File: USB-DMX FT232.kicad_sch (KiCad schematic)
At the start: 26 parts, among them J1 USB, J2 NC3MAFH-PH, U1 FT232RL, U2 TEA1-0505, U3 6N137, U4 MAX485E

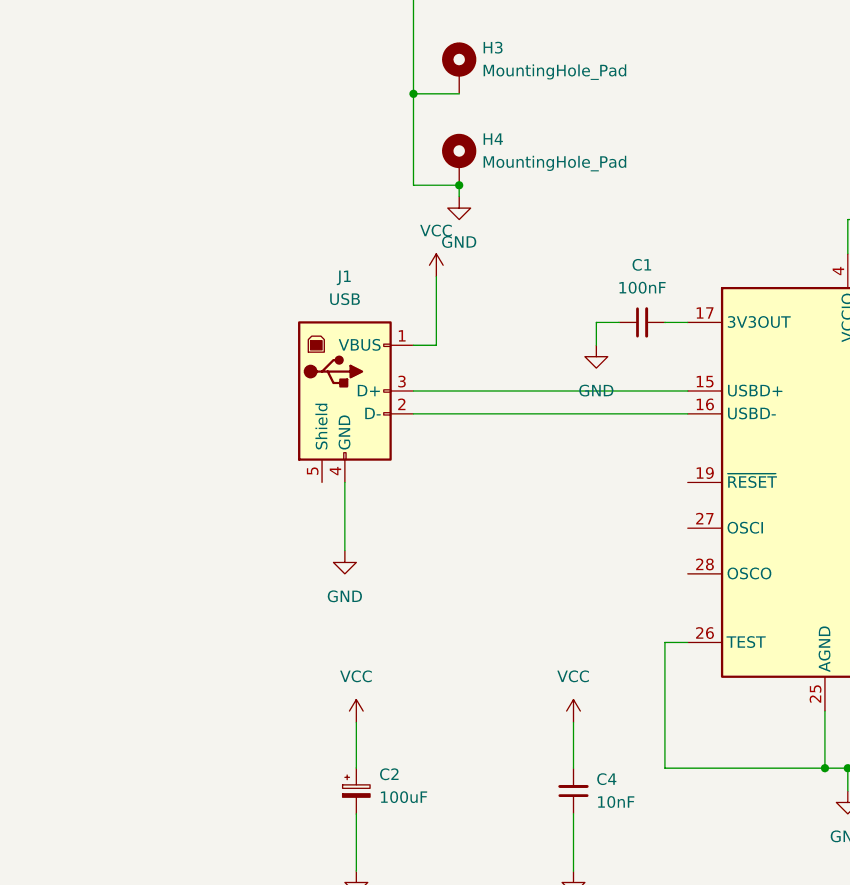
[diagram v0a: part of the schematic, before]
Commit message: usbc version
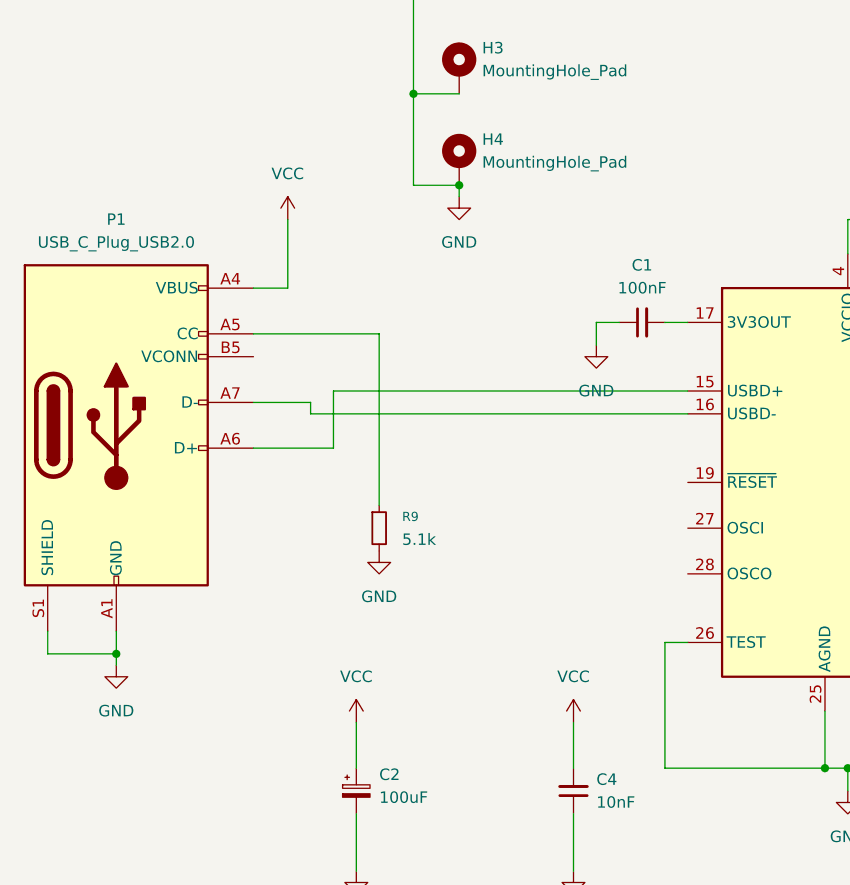
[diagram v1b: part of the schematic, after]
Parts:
- removed J1: USB, Connector_USB:USB_B_Lumberg_2411_02_Horizontal, symbol Connector:USB_B
- added P1: USB_C_Plug_USB2.0, Connector_USB:USB_C_Receptacle_JAE_DX07S016JA1R1500, symbol Connector:USB_C_Plug_USB2.0
- added R9: 5.1k, Resistor_SMD:R_0805_2012Metric_Pad1.20x1.40mm_HandSolder, symbol Device:R_Small
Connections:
- net GND: now also P1.A1 (GND), P1.A12 (GND), P1.B1 (GND), P1.B12 (GND), P1.S1 (SHIELD), R9.2
- net VCC: now also P1.A4 (VBUS), P1.A9 (VBUS), P1.B4 (VBUS), P1.B9 (VBUS)
- net at U1.16 (USBD-): now also P1.A7 (D-)
- net at U1.15 (USBD+): now also P1.A6 (D+)
- new net: P1.A5 (CC), R9.1
